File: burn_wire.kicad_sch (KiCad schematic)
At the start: 13 parts, among them Q4 Q_PI, Q5 TIP122, Q6 Q_NPN_BEC

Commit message: Updated files and include work done for PCB
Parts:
- D7: footprint (none) -> LED_SMD:LED_0603_1608Metric
- F3: footprint (none) -> Fuse:Fuse_1812_4532Metric
- Q4, Q6: footprint (none) -> Package_TO_SOT_SMD:SOT-23
- R10, R11, R12, R13, R14, R21, R8: footprint (none) -> Resistor_SMD:R_0201_0603Metric
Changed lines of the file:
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@@
 			)
 		)
-		(property "Footprint" ""
+		(property "Footprint" "Fuse:Fuse_1812_4532Metric"
 			(at 78.74 56.642 90)
 			(effects
@@
 			)
 		)
-		(property "Footprint" ""
+		(property "Footprint" "Resistor_SMD:R_0201_0603Metric"
 			(at 64.516 88.646 90)
 			(effects
@@
 			)
 		)
-		(property "Footprint" ""
+		(property "Footprint" "Resistor_SMD:R_0201_0603Metric"
 			(at 124.714 77.724 90)
 			(effects
@@
 			)
 		)
-		(property "Footprint" ""
+		(property "Footprint" "Package_TO_SOT_SMD:SOT-23"
 			(at 91.44 78.74 0)
 			(effects
@@
 			)
 		)
-		(property "Footprint" ""
+		(property "Footprint" "LED_SMD:LED_0603_1608Metric"
 			(at 137.16 78.74 0)
 			(effects
@@
 			)
 		)
-		(property "Footprint" ""
+		(property "Footprint" "Resistor_SMD:R_0201_0603Metric"
 			(at 64.516 83.566 90)
 			(effects
@@
 			)
 		)
-		(property "Footprint" ""
+		(property "Footprint" "Resistor_SMD:R_0201_0603Metric"
 			(at 96.266 59.436 90)
 			(effects
@@
 			)
 		)
-		(property "Footprint" ""
+		(property "Footprint" "Resistor_SMD:R_0201_0603Metric"
 			(at 77.216 93.726 90)
 			(effects
@@
 			)
 		)
-		(property "Footprint" ""
+		(property "Footprint" "Resistor_SMD:R_0201_0603Metric"
 			(at 96.774 98.806 90)
 			(effects
@@
 			)
 		)
-		(property "Footprint" ""
+		(property "Footprint" "Package_TO_SOT_SMD:SOT-23"
 			(at 77.47 72.39 0)
 			(effects
@@
 			)
 		)
-		(property "Footprint" ""
+		(property "Footprint" "Resistor_SMD:R_0201_0603Metric"
 			(at 55.626 99.314 90)
 			(effects

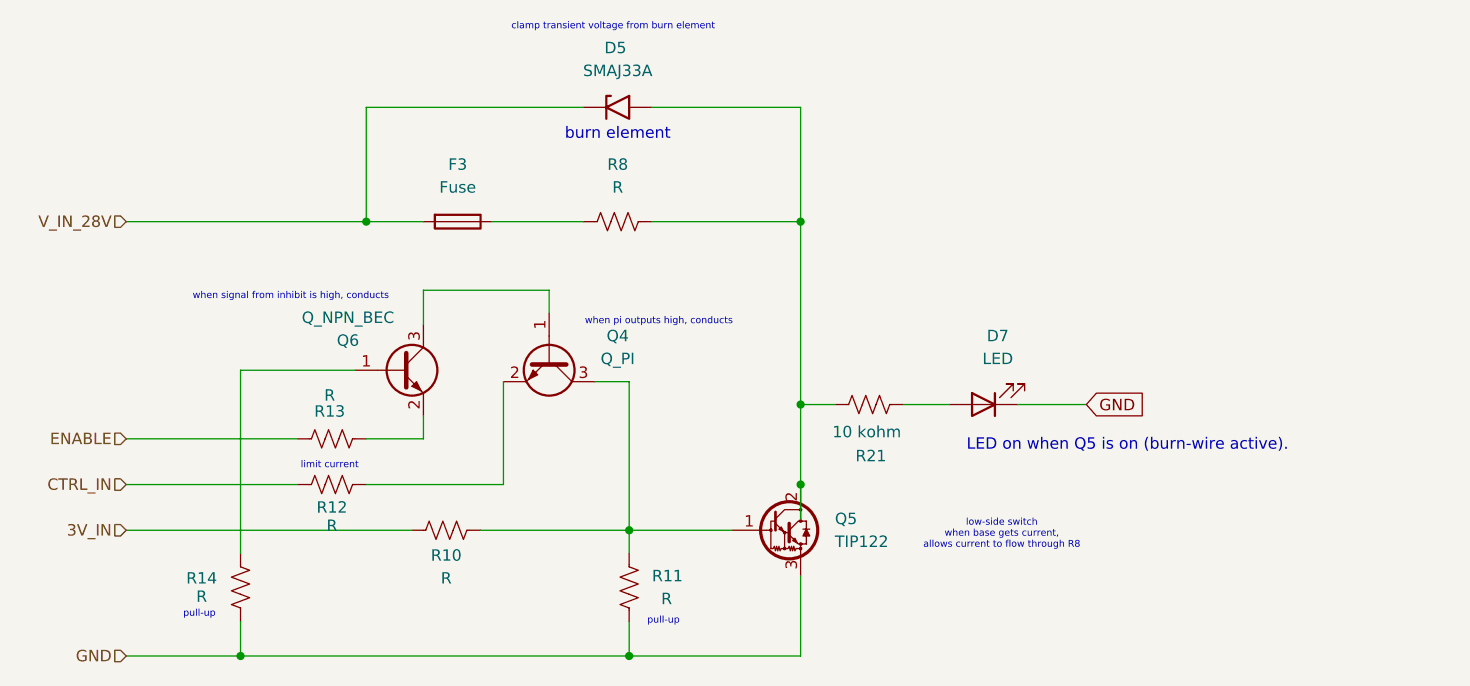
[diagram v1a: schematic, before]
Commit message: PCB is mostly laid out, routing is WIP
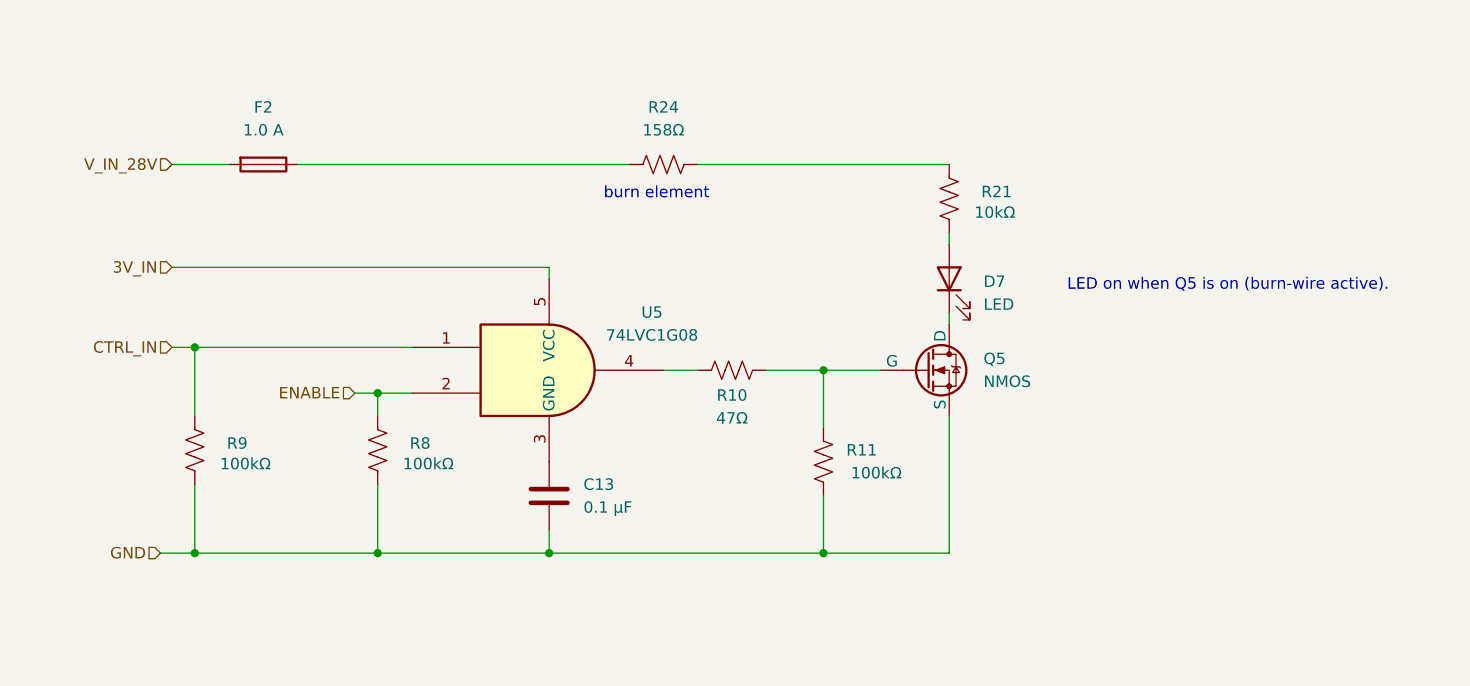
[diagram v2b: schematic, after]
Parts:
- removed D5: SMAJ33A, Diode_SMD:D_SMA, symbol Diode:SMAJ33A
- removed F3: Fuse, Fuse:Fuse_1812_4532Metric, symbol Device:Fuse
- removed Q4: Q_PI, Package_TO_SOT_SMD:SOT-23, symbol Transistor_BJT:Q_NPN_BEC
- removed Q5: TIP122, Package_TO_SOT_THT:TO-220-3_Vertical, symbol Transistor_BJT:TIP122
- removed Q6: Q_NPN_BEC, Package_TO_SOT_SMD:SOT-23, symbol Transistor_BJT:Q_NPN_BEC
- removed R12, R13, R14: R, Resistor_SMD:R_0201_0603Metric, symbol Device:R_US
- added C13: 0.1 µF, Capacitor_SMD:C_0603_1608Metric, symbol Device:C
- added F2: 1.0 A, Fuse:Fuse_1812_4532Metric, symbol Device:Fuse
- added Q5: NMOS, Package_TO_SOT_SMD:SOT-23, symbol Simulation_SPICE:NMOS
- added R24: 158Ω, Resistor_SMD:R_0201_0603Metric, symbol Device:R_US
- added R9: 100kΩ, Resistor_SMD:R_0201_0603Metric, symbol Device:R_US
- added U5: 74LVC1G08, Package_TO_SOT_SMD:SOT-23-5, symbol 74xGxx:74LVC1G08
- R10: value R -> 47Ω
- R11, R8: value R -> 100kΩ
- R21: value 10 kohm -> 10kΩ
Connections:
- net 3V_IN: now also U5.5 (VCC); no longer R10.2
- net CTRL_IN: now also R9.1, U5.1
- net ENABLE: now also R8.1, U5.2
- net GND: now also R8.2, C13.2, Q5.3 (S), R9.2; no longer D7.1 (K)
- net V_IN_28V: now also F2.2
- net at R21.1: now also R24.1; no longer R8.1
- net at R10.1, R11.2: now also Q5.2 (G)
- new net: D7.1 (K), Q5.1 (D)
- new net: C13.1, U5.3 (GND)
- new net: R10.2, U5.4
- new net: F2.1, R24.2
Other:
- note removed: "clamp transient voltage from burn element"
- note removed: "limit current"
- note removed: "low-side switch when base gets current, allows current to flow through R8"
- note removed: "pull-up"
- note removed: "when pi outputs high, conducts"
- note removed: "when signal from inhibit is high, conducts"
